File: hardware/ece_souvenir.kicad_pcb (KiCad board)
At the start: 2 copper layers, 30 x 30 mm, 38 parts, among them U1 TLC555CDR

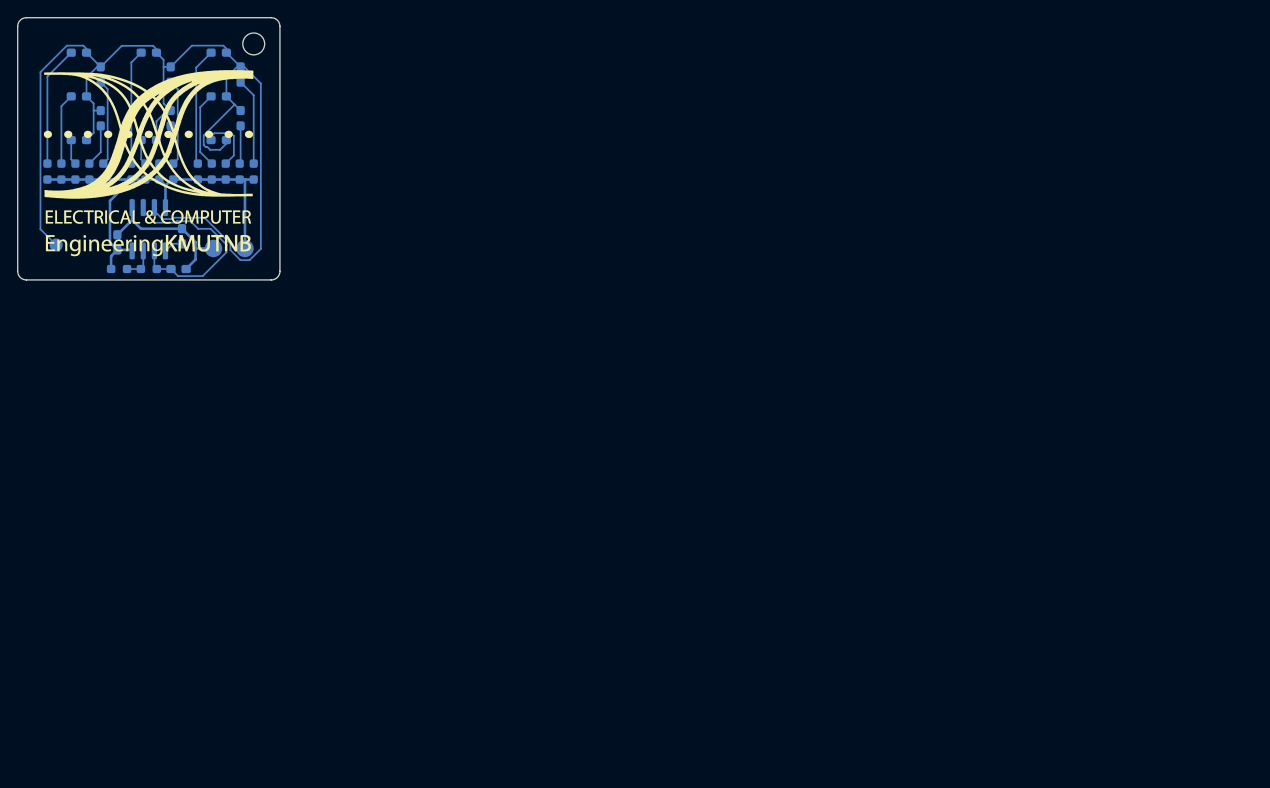
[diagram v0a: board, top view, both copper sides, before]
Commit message: chore(pcb): board moved onto drawing sheet in KiCad (user edit)
Whole board translated by (+111.1825, +56.0585) mm; no other change
(148 segments, 38 footprints, identical relative geometry).

Co-Authored-By: Claude Opus 5.5 <noreply@anthropic.com>
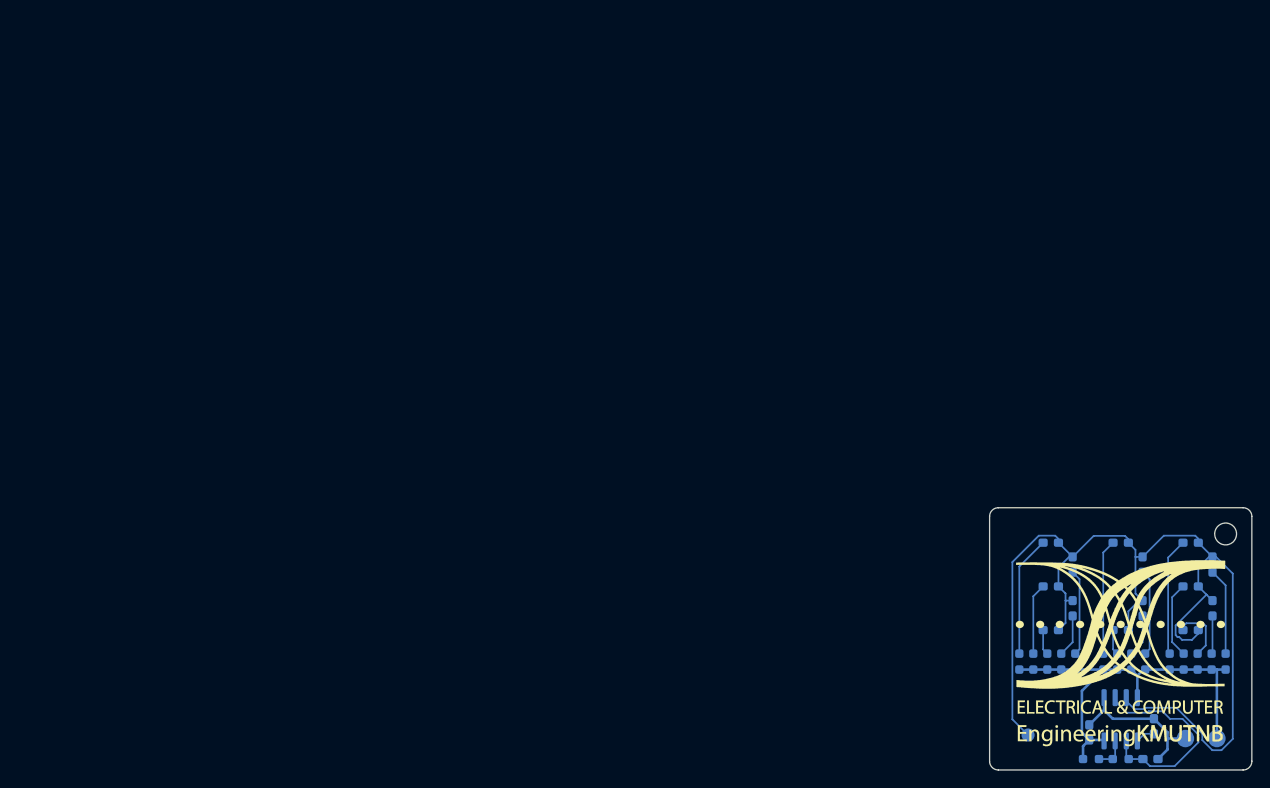
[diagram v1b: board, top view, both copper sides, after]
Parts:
- moved C1 124.5 mm to (129.6, 84.8)
- moved D1 124.5 mm to (134.2, 60.1)
- moved D10 124.5 mm to (118.2, 60.1)
- moved D11 124.5 mm to (120.7, 62.6)
- moved D12 124.5 mm to (118.2, 65.1)
- moved D13 124.5 mm to (120.7, 67.6)
- moved D14 124.5 mm to (118.2, 70.1)
- moved D2 124.5 mm to (136.7, 62.6)
- moved D3 124.5 mm to (134.2, 65.1)
- moved D4 124.5 mm to (136.7, 67.6)
- moved D5 124.5 mm to (134.2, 70.1)
- moved D6 124.5 mm to (126.2, 60.1)
- moved D7 124.5 mm to (128.7, 62.6)
- moved D8 124.5 mm to (128.7, 67.6)
- moved D9 124.5 mm to (126.2, 70.1)
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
